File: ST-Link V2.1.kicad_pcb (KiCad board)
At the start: 2 copper layers, 44 parts, among them J1 Conn_01x08, J2 USB_OTG, J3 Conn_01x06, J4 Conn_01x08, Q1 MMBT3904, U0 stm32, U1 MIC5219-3.3, U2 USBLC6-2SC6, X1 8MHz

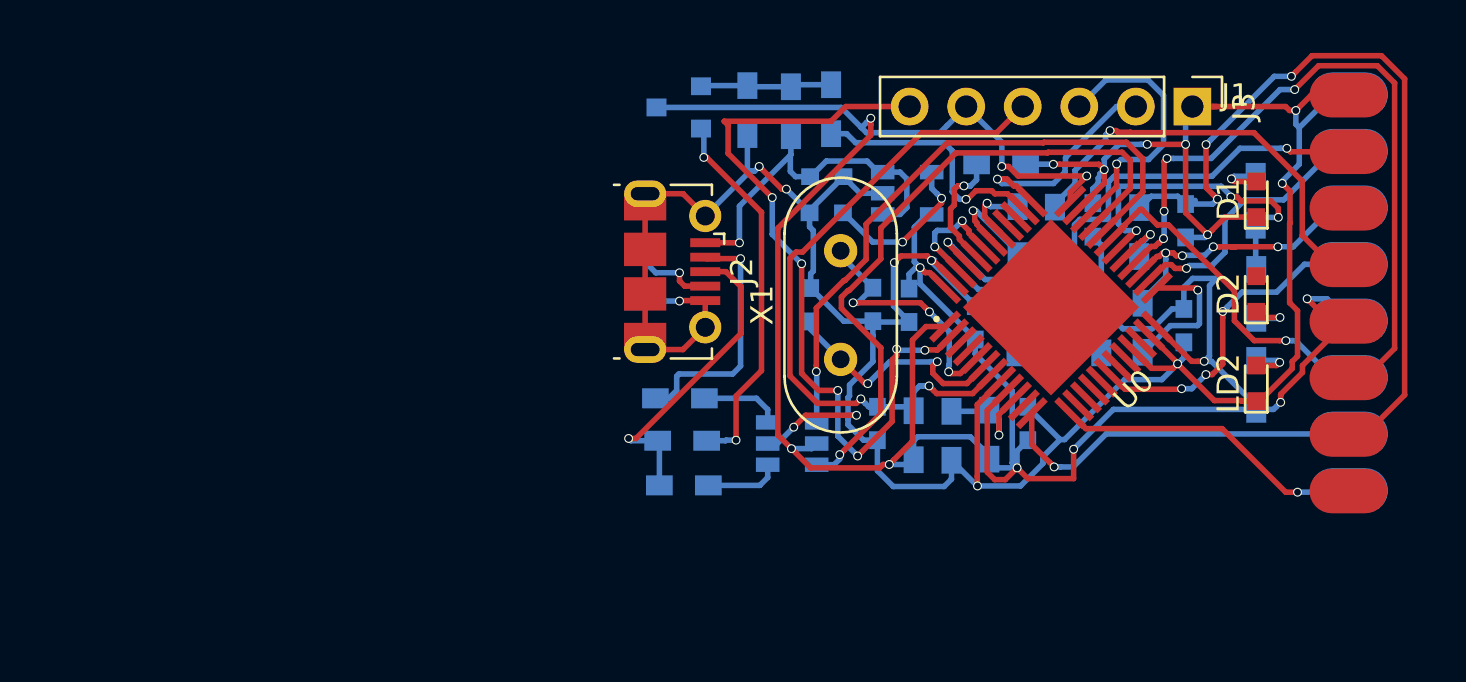
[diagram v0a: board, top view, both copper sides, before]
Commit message: working footprint(need to reroute)
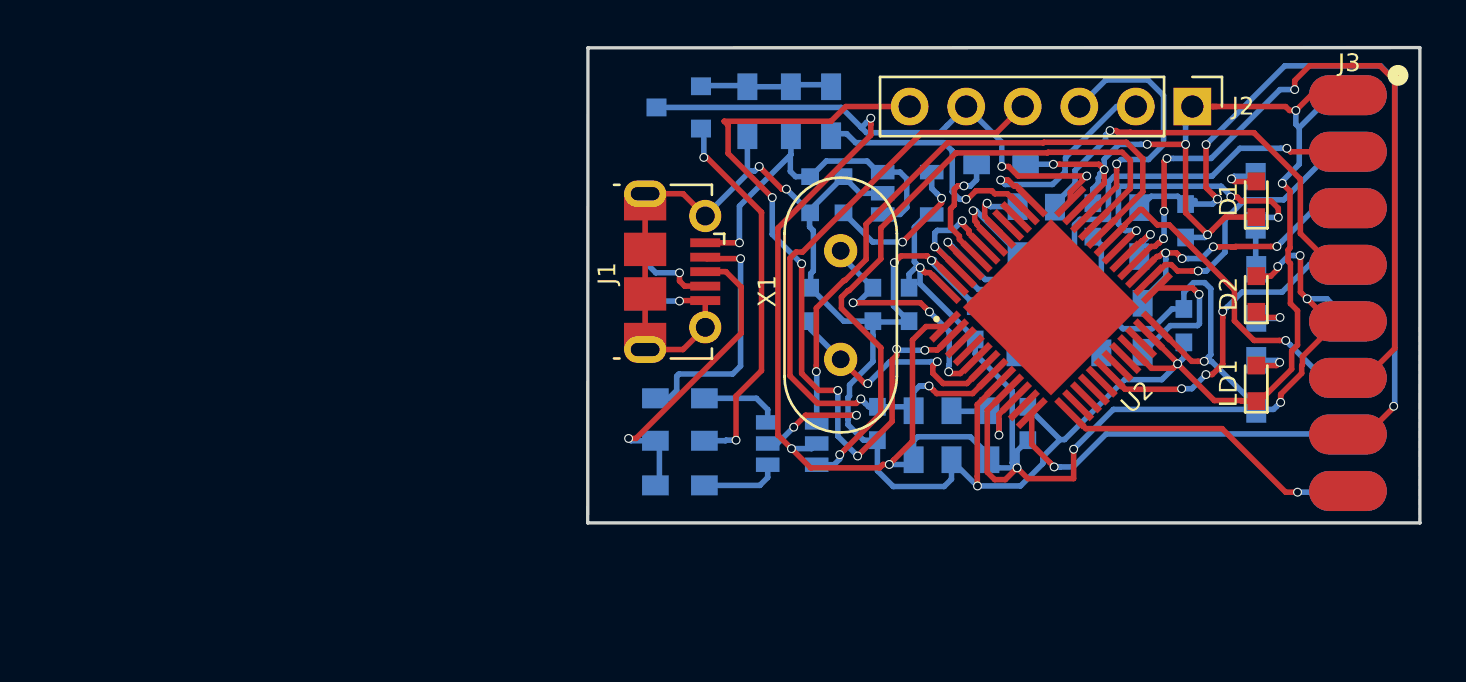
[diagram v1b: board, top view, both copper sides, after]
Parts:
- removed the J1 at (168.7, 94.6)
- added J3: Conn_01x08, MetalPad:METAL_PAD, F.Cu at (168.7, 94.6)
- moved R4 0.18 mm to (138.7, 112.1)
- moved R6 0.10 mm to (138.7, 110.1)
- moved R11 0.09 mm to (145.4, 95.3)
- moved J4 0.05 mm to (168.7, 94.6)
- moved R9 0.05 mm to (141.7, 95.3)
- renumbered C18 to C1, C13 to C10, C7 to C2, C6 to C3, C15 to C4, C17 to C5, C8 to C6, C16 to C7, C5 to C8, C14 to C9, J2 to J1, J3 to J2, LD2 to LD1, R31 to R1, R14 to R10, R10 to R11, R3 to R12, R2 to R13, R11 to R14, R22 to R15, R4 to R16, R20 to R17, R21 to R18, R12 to R19, R29 to R2, R13 to R20, R19 to R21, R30 to R3, R7 to R4, R8 to R5, R5 to R7, R9 to R8, R23 to R9, U2 to U1, U0 to U2, U1 to U3
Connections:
- D2 pad 2: Net-(D2-Pad2) -> /3V3_ST_LINK
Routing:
- net /3V3_ST_LINK: track 130.3 -> 133.1 mm, vias 11 -> 13
- added copper zone on F.Cu, net /3V3_ST_LINK
- added copper zone on B.Cu, net GND
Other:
- board outline added: 37.4 x 21.3 mm

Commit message: routing
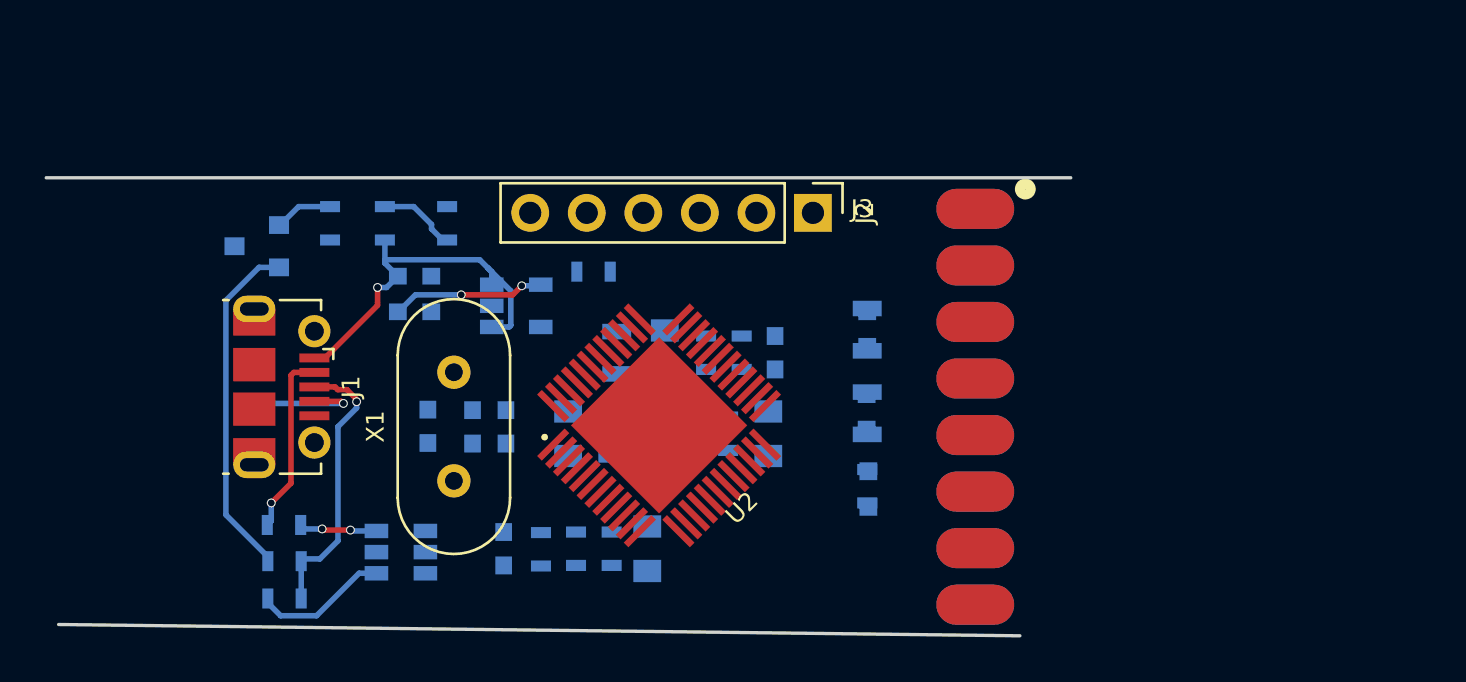
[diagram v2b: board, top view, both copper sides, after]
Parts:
- removed LD1: LED,RED, LEDs:LED_0603
- added D3: LED, LEDs:LED_0603, B.Cu at (147.1, 112.3)
- C4, C5, C6, C8: footprint Capacitors_SMD:C_0603 -> Capacitors_SMD:C_0805
- D1, D2: moved to B.Cu
- R1, R10, R11, R14, R15, R16, R19, R2, R20, R21, R3, R4, R5, R6, R7, R8, R9: footprint Resistors_SMD:R_0603_HandSoldering -> Resistors_SMD:R_0603
- R12, R13, R17, R18: footprint Resistors_SMD:R_0603_HandSoldering -> Resistors_SMD:R_0805
- moved C5 20.1 mm to (138.0, 106.2), turned to 270 degrees
- moved Q1 20.0 mm to (119.6, 101.4)
- moved R9 19.4 mm to (122.9, 100.3)
- moved C7 19.4 mm to (142.9, 106.2), turned to 90 degrees
- moved C8 19.3 mm to (142.6, 109.8)
- moved R3 19.3 mm to (134.0, 115.0)
- moved R14 19.2 mm to (140.8, 109.8)
- moved R19 19.1 mm to (139.1, 109.8)
- moved C9 19.0 mm to (126.7, 102.7)
- moved C10 19.0 mm to (126.7, 104.3), turned to 0 degrees
- moved C6 19.0 mm to (133.6, 109.8)
- moved R10 18.9 mm to (134.8, 102.5)
- moved C11 18.9 mm to (130.8, 109.5)
- moved R8 18.9 mm to (125.4, 100.3)
- moved R20 18.8 mm to (137.4, 109.8)
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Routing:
- net GND: track 143.6 -> 0.00 mm, vias 16 -> 0
- net /3V3_ST_LINK: track 133.1 -> 0.00 mm, vias 13 -> 0
- net /MCO: track 35.4 -> 0.00 mm, vias 3 -> 0
- net /PC13: track 35.0 -> 0.00 mm, vias 6 -> 0
- net /PWR_ENn: track 32.6 -> 0.00 mm, vias 4 -> 0
- net /USB_DP: track 30.1 -> 0.00 mm, vias 1 -> 0
- net /NRST: track 29.9 -> 0.00 mm, vias 2 -> 0
- net /USB_DM: track 28.2 -> 0.00 mm, vias 1 -> 0
- net /T_RESET: track 19.1 -> 0.00 mm, vias 1 -> 0
- net /T_SWIM: track 18.7 -> 0.00 mm, vias 1 -> 0
- net /STLINK_TX: track 16.7 -> 0.00 mm, vias 1 -> 0
- net /T_SWO: track 15.3 -> 0.00 mm, vias 1 -> 0
- net /LED_STLINK: track 15.0 -> 0.00 mm, vias 3 -> 0
- net /T_NRST: track 14.8 -> 0.00 mm, vias 3 -> 0
- net /STLINK_RX: track 14.0 -> 0.00 mm, vias 1 -> 0
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- removed copper zone on F.Cu, net /3V3_ST_LINK
- removed copper zone on B.Cu, net GND
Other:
- board size 37.4 x 21.3 mm -> 46 x 20.6 mm
